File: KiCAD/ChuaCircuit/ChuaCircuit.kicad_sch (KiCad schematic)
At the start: 16 parts, among them U1 TL084

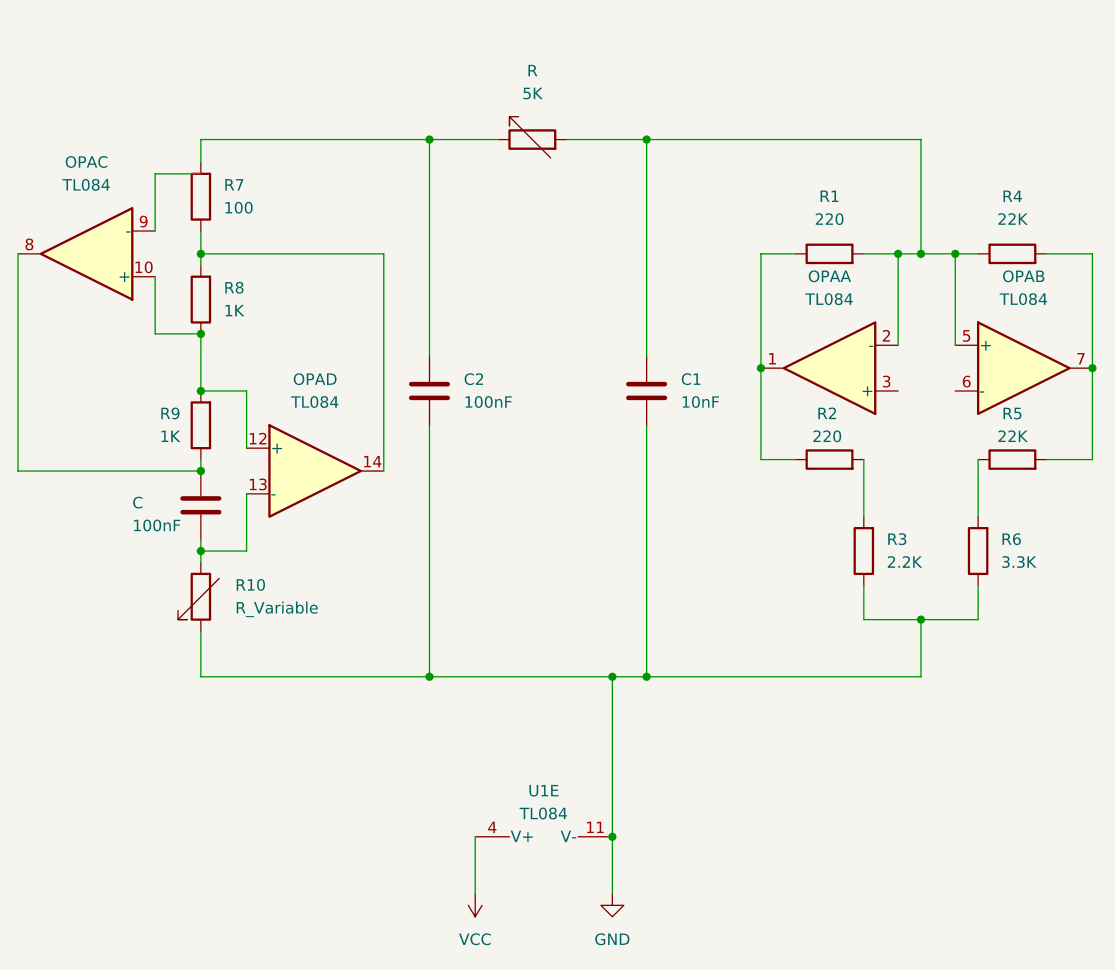
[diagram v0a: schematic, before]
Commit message: Finished schematic, need to add footprints for parts tho
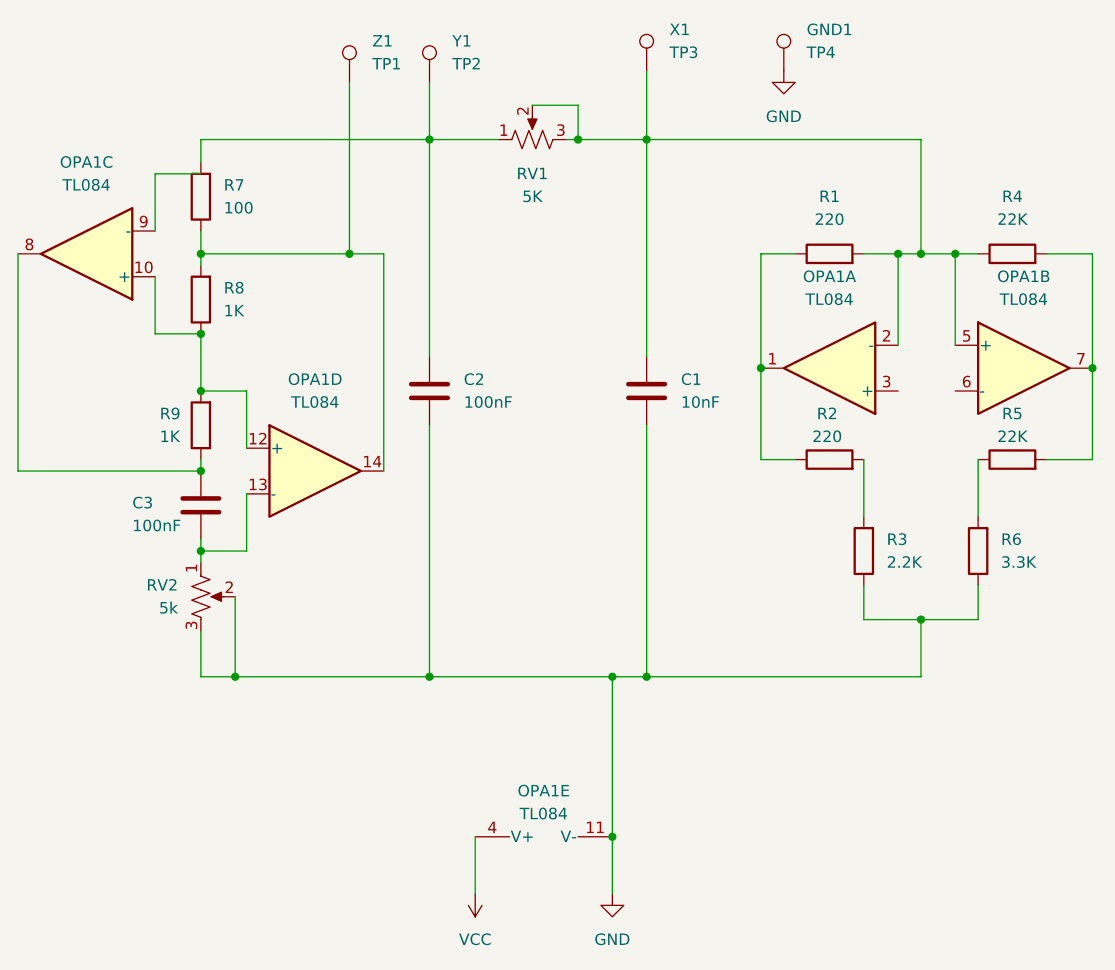
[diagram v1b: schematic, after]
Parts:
- removed unit 3 of OPA
- removed R: 5K, symbol Device:R_Variable
- removed R10: R_Variable, symbol Device:R_Variable
- added GND1: TP4, symbol Connector:TestPoint
- added unit 3 of OPA1
- added RV1: 5K, Connector_PinHeader_2.54mm:PinHeader_1x03_P2.54mm_Vertical, symbol Device:R_Potentiometer_US
- added RV2: 5k, Connector_PinHeader_2.54mm:PinHeader_1x03_P2.54mm_Vertical, symbol Device:R_Potentiometer_US
- added X1: TP3, symbol Connector:TestPoint
- added Y1: TP2, symbol Connector:TestPoint
- added Z1: TP1, symbol Connector:TestPoint
- OPA1: renamed from OPA; footprint (none) -> SamacSys_Parts:TL084
- R1, R2, R3, R4, R5, R6, R7, R8, R9: footprint (none) -> Resistor_SMD:R_0201_0603Metric
- renumbered C to C3, OPA to OPA1, U1 to OPA1
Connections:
- net GND: now also GND1.1, RV2.2, RV2.3
- net at C1.1, OPA1.2 (-), OPA1.5 (+)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: now also RV1.2, RV1.3, X1.1
- net at OPA1.12 (+), R8.1, R9.2: now also OPA1.10 (+)
- net at OPA1.14, R7.1, R8.2: now also Z1.1
- net at C2.1, R7.2: now also RV1.1, Y1.1
- net at C3.1, R9.1: now also OPA1.8
- net at C3.2, OPA1.13 (-): now also RV2.1
